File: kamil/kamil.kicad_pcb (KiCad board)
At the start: 2 copper layers, 98.6 x 45.1 mm, 33 parts, among them J1 RELAY, J2 RELAY OUTPUT, J3 CC1101, J4 DEBUG INTERFACE, J5 230AC, J6 LED, Q2 2N7000, SW1 SW_Push, U1 LNK304P, U2 AMS1117-3.3, U3 STM32G030F6Px

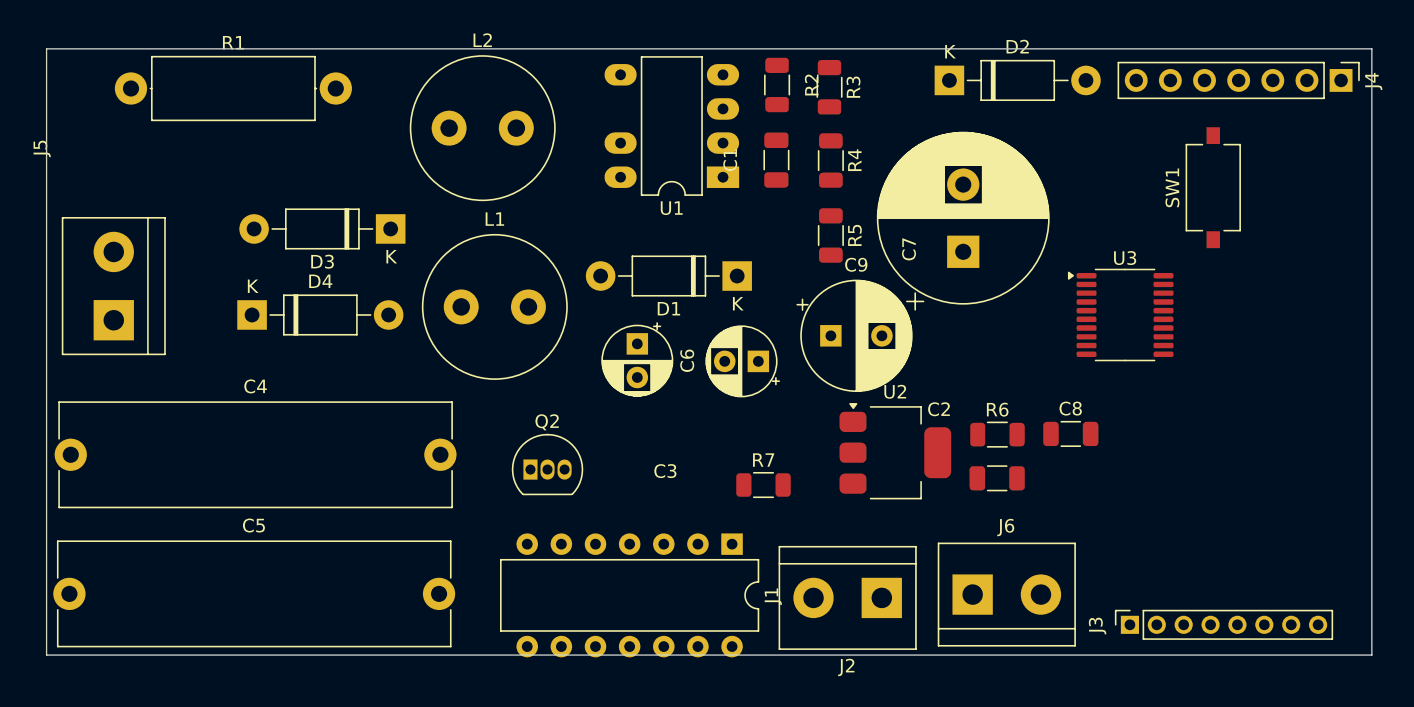
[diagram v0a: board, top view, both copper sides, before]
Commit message: To be continued.
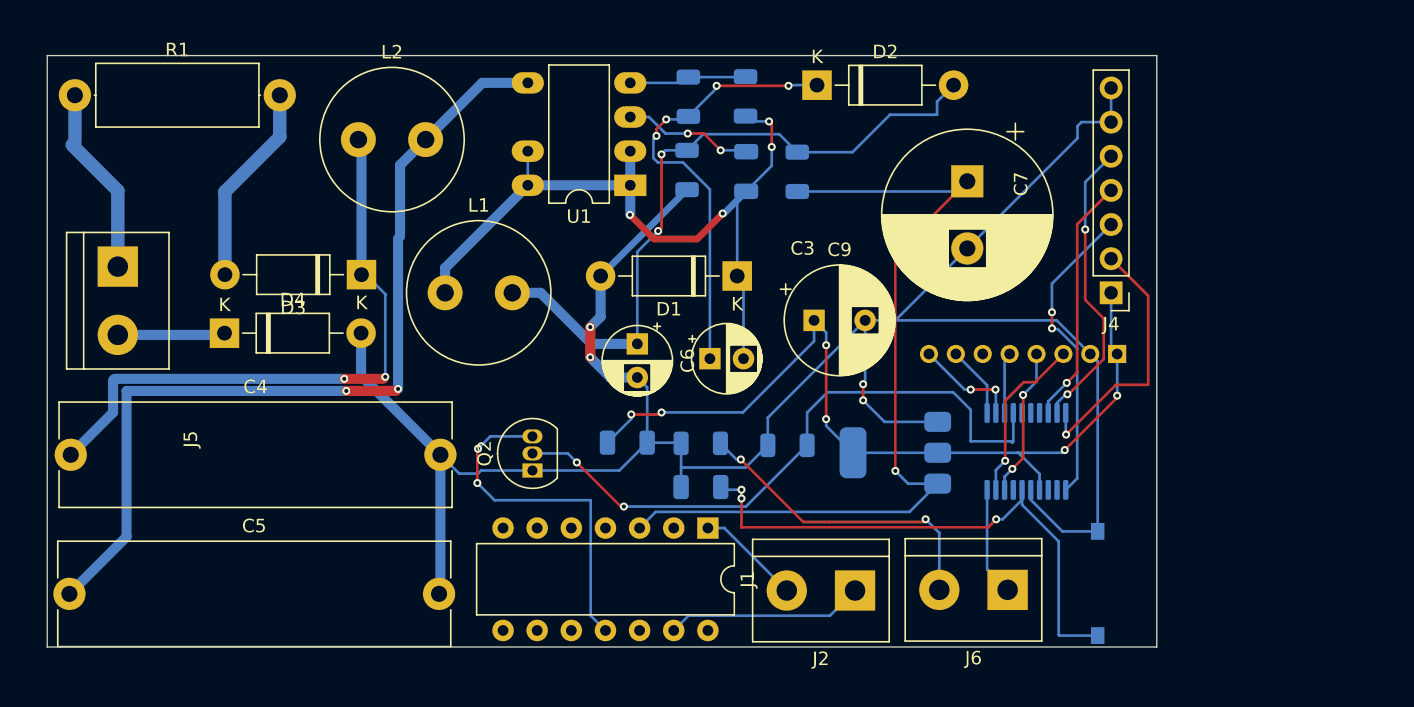
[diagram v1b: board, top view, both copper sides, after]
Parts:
- C1, C2, C8, J3, R2, R3, R4, R5, R6, R7, SW1, U2, U3: moved to B.Cu
- moved C8 33.0 mm to (64.4, 54.0), turned to 180 degrees
- moved SW1 30.7 mm to (99.4, 64.5), turned to -90 degrees
- moved J4 23.3 mm to (100.4, 42.9), turned to 180 degrees
- moved R6 22.1 mm to (69.9, 54.0), turned to 180 degrees
- moved C2 22.1 mm to (69.9, 57.3), turned to 180 degrees
- moved J3 20.2 mm to (100.8, 47.4)
- moved U3 12.5 mm to (94.1, 54.6), turned to 90 degrees
- moved R4 10.7 mm to (68.8, 33.7)
- moved R3 10.5 mm to (69.0, 28.3)
- moved D2 9.86 mm to (78.5, 27.4)
- moved U1 6.93 mm to (64.6, 34.9)
- moved L2 6.80 mm to (44.4, 31.4)
- moved R5 5.36 mm to (77.0, 33.9)
- moved C7 5.26 mm to (89.7, 34.5), turned to -90 degrees
- moved R1 4.20 mm to (23.3, 28.1)
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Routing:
- net GND: track 0.00 -> 164.1 mm, vias 0 -> 4
- net Net-(U1-D): track 0.00 -> 65.9 mm, vias 0 -> 2
- net +3.3V: track 0.00 -> 64.1 mm, vias 0 -> 6
- net +5V: track 0.00 -> 63.8 mm, vias 0 -> 1
- net Net-(D1-K): track 0.00 -> 57.2 mm, vias 0 -> 4
- net Net-(D2-A): track 0.00 -> 51.3 mm, vias 0 -> 2
- net Net-(Q2-G): track 0.00 -> 47.5 mm, vias 0 -> 2
- net Net-(D3-K): track 0.00 -> 45.9 mm, vias 0 -> 2
- net Net-(U3-NRST): track 0.00 -> 41.7 mm, vias 0 -> 3
- net Net-(D2-K): track 0.00 -> 33.4 mm, vias 0 -> 4
- net Net-(J1-Pin_11): track 0.00 -> 26.1 mm, vias 0 -> 2
- net Net-(J6-Pin_2): track 0.00 -> 23.4 mm, vias 0 -> 2
- net Net-(J4-Pin_3): track 0.00 -> 22.9 mm, vias 0 -> 2
- net Net-(J4-Pin_5): track 0.00 -> 22.0 mm, vias 0 -> 2
- net Net-(J4-Pin_2): track 0.00 -> 19.8 mm, vias 0 -> 1
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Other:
- board size 98.6 x 45.1 mm -> 82.5 x 44 mm
